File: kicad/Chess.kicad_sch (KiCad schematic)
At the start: 71 parts, among them J2 Conn_01x08_Pin, U1 CD74HC4067M, U12 A1302xUA, U13 A1302xUA, U14 A1302xUA, U15 A1302xUA, U16 A1302xUA, U17 A1302xUA, U18 A1302xUA, U19 A1302xUA, U2 ADS1015IDGS, U20 A1302xUA, U21 A1302xUA, U22 A1302xUA, U23 A1302xUA, U24 A1302xUA, U25 A1302xUA, U26 A1302xUA, U27 A1302xUA, U28 A1302xUA, U29 A1302xUA, U3 MP1584EN, U30 A1302xUA, U31 A1302xUA, U32 A1302xUA, U33 A1302xUA, U34 A1302xUA, U35 A1302xUA, U36 A1302xUA, U37 A1302xUA, U38 A1302xUA, U39 A1302xUA, U4 CD74HC4067M, U40 A1302xUA, U41 A1302xUA, U42 A1302xUA, U43 A1302xUA, U44 A1302xUA, U45 A1302xUA, U46 A1302xUA, U47 A1302xUA, U48 A1302xUA, U49 A1302xUA, U5 CD74HC4067M, U50 A1302xUA, U51 A1302xUA, U52 A1302xUA, U53 A1302xUA, U54 A1302xUA, U55 A1302xUA, U56 A1302xUA, U57 A1302xUA, U58 A1302xUA, U59 A1302xUA, U6 CD74HC4067M, U60 A1302xUA, U61 A1302xUA, U62 A1302xUA, U63 A1302xUA, U64 A1302xUA, U65 A1302xUA, U66 A1302xUA, U67 A1302xUA, U68 A1302xUA, U69 A1302xUA, U70 A1302xUA, U71 A1302xUA, U72 A1302xUA, U73 A1302xUA, U74 A1302xUA, U75 A1302xUA

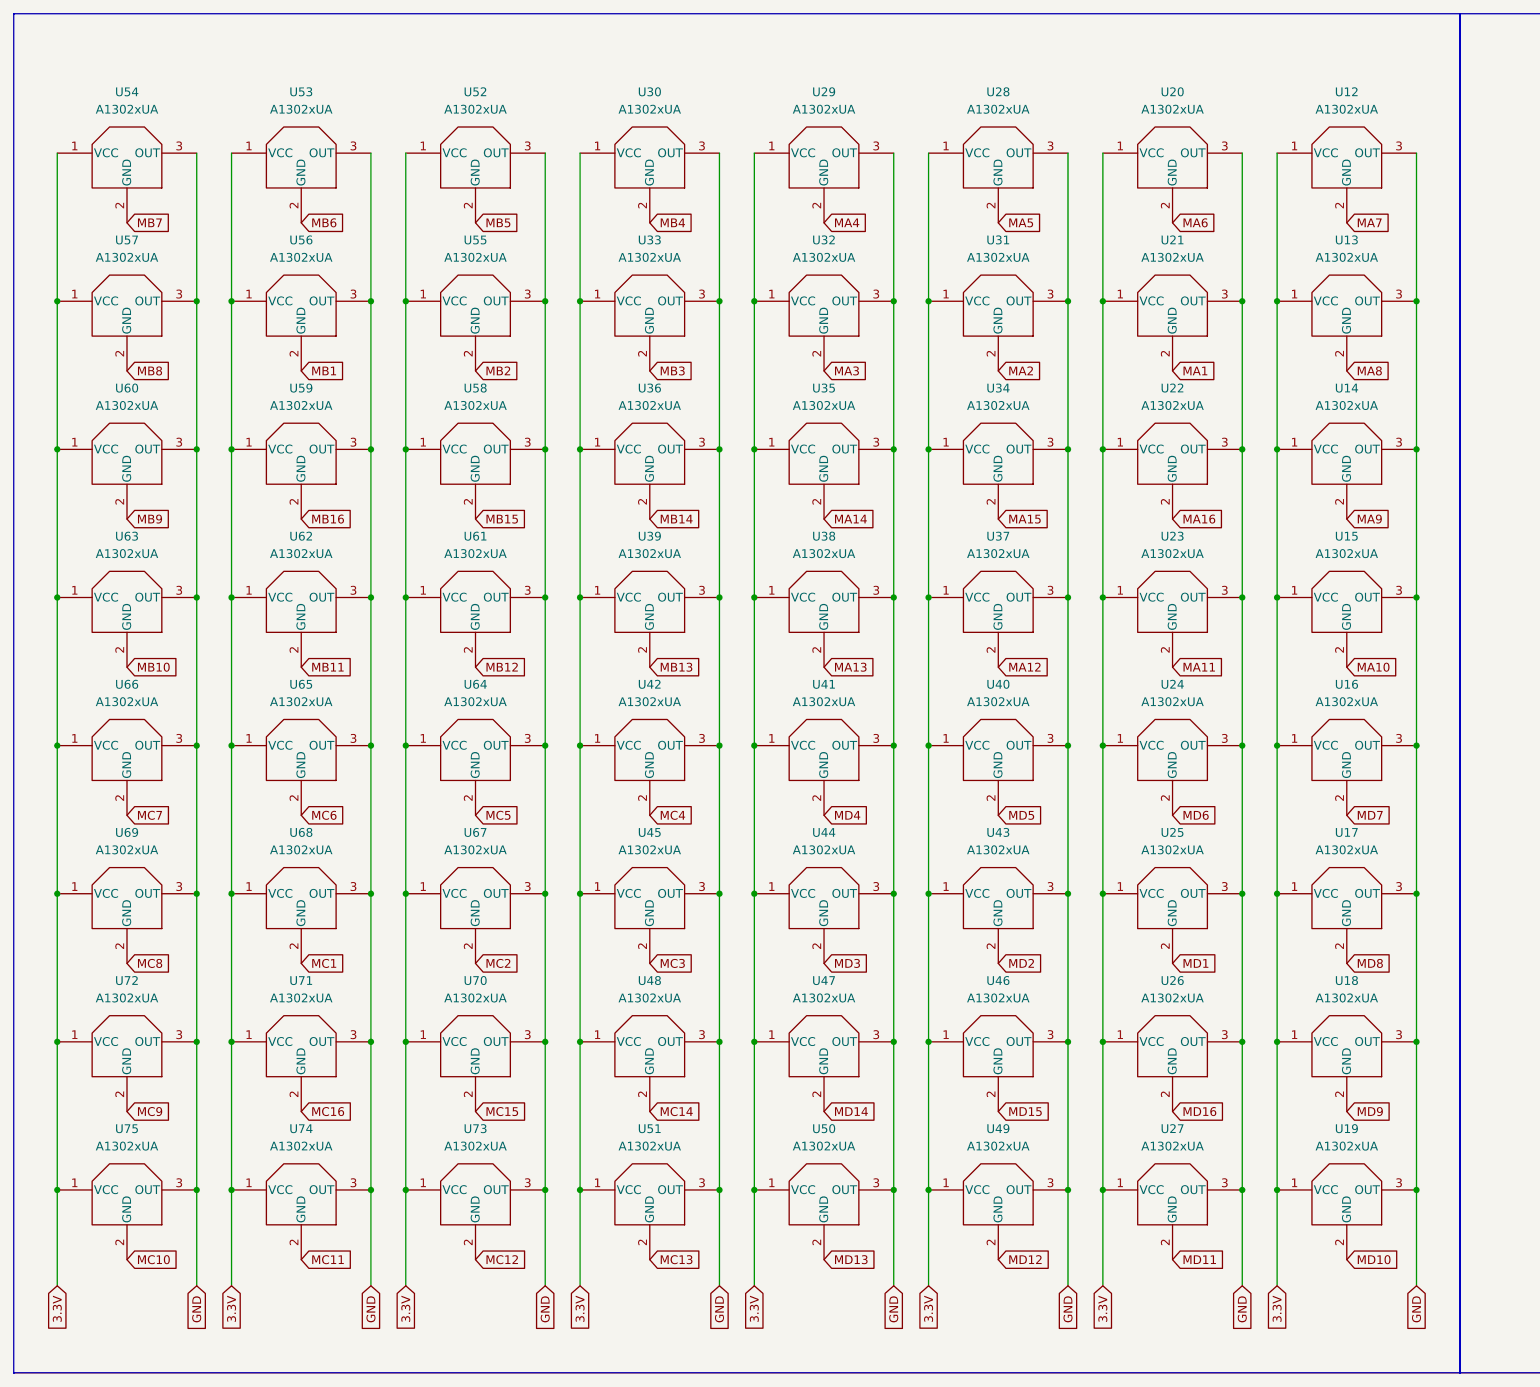
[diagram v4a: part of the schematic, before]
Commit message: fixes
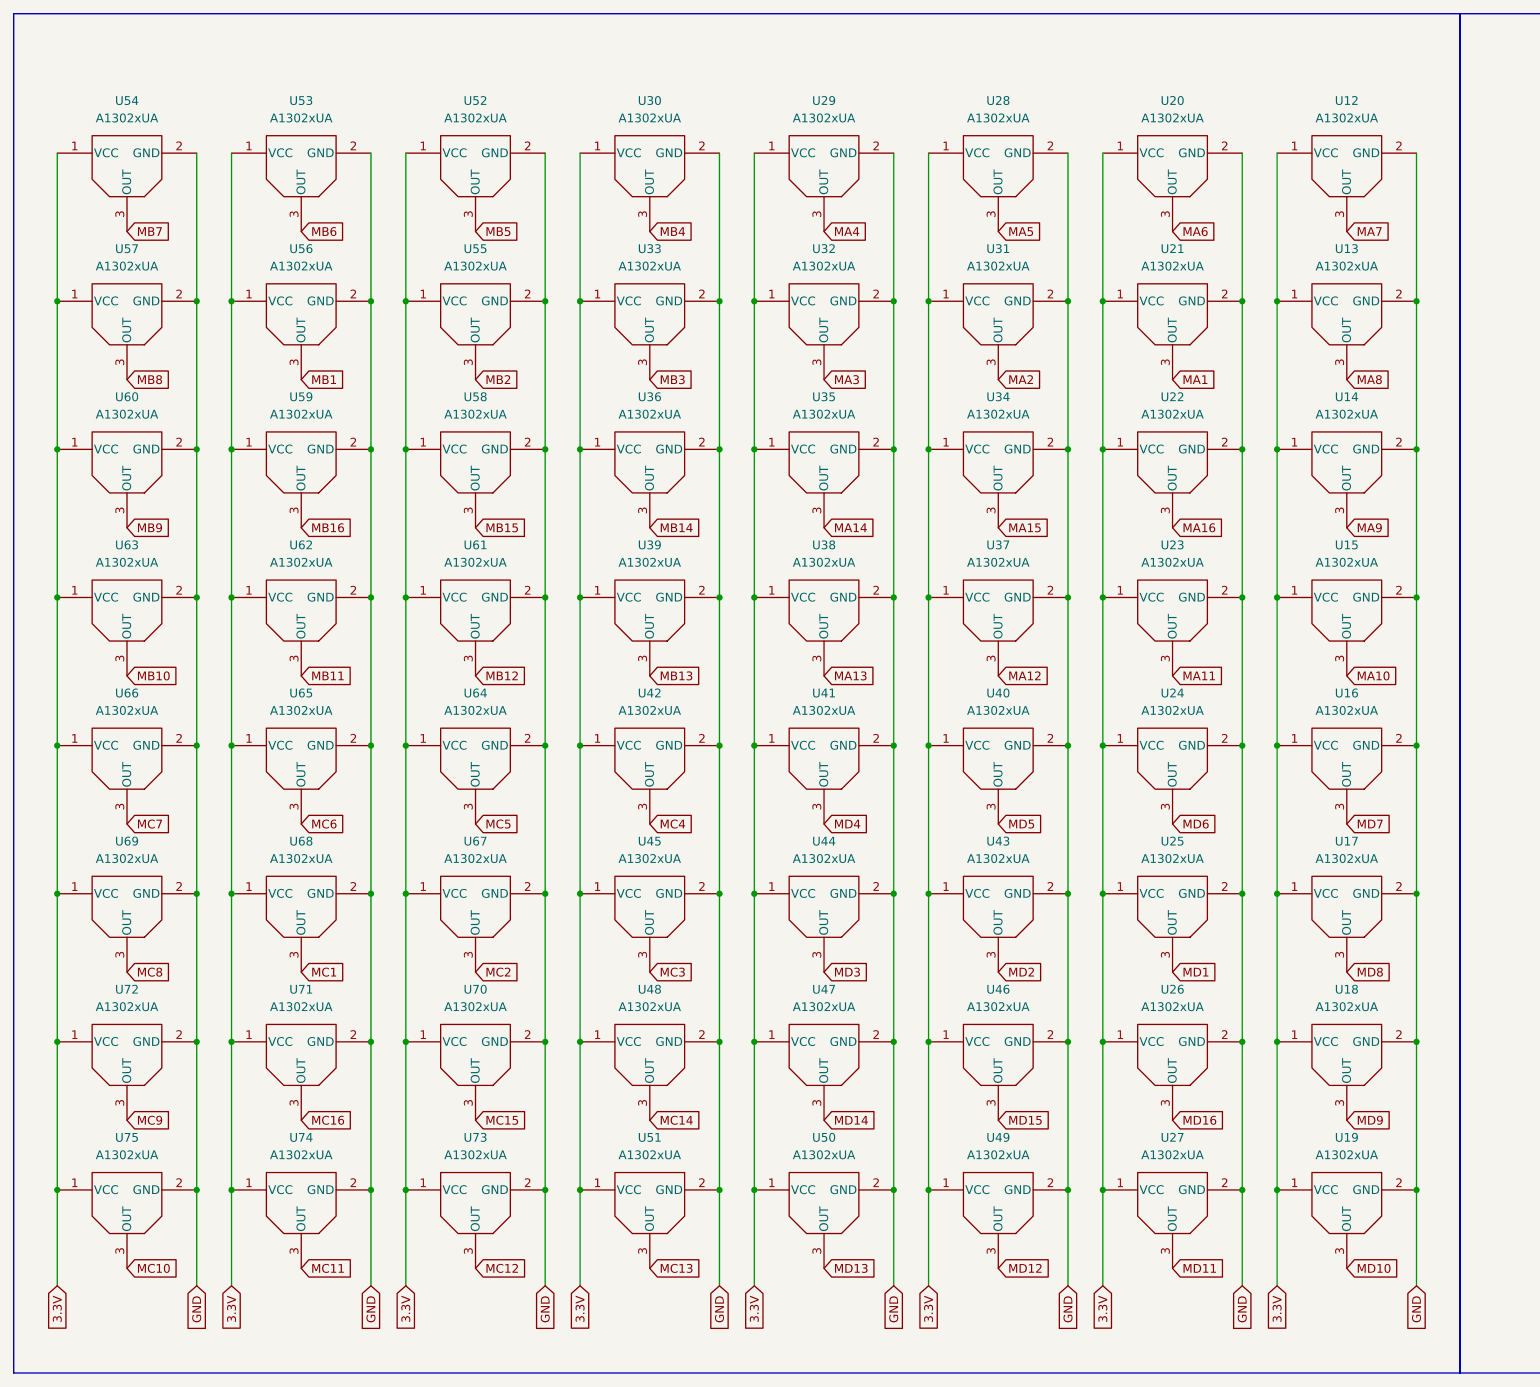
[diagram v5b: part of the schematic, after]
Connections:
- net GND: now also U12.2 (GND), U13.2 (GND), U14.2 (GND), U15.2 (GND), U16.2 (GND), U17.2 (GND), U18.2 (GND), U19.2 (GND), U20.2 (GND), U21.2 (GND), U22.2 (GND), U23.2 (GND), U24.2 (GND), U25.2 (GND), U26.2 (GND), U27.2 (GND), U28.2 (GND), U29.2 (GND), U30.2 (GND), U31.2 (GND), U32.2 (GND), U33.2 (GND), U34.2 (GND), U35.2 (GND), U36.2 (GND), U37.2 (GND), U38.2 (GND), U39.2 (GND), U40.2 (GND), U41.2 (GND), U42.2 (GND), U43.2 (GND), U44.2 (GND), U45.2 (GND), U46.2 (GND), U47.2 (GND), U48.2 (GND), U49.2 (GND), U50.2 (GND), U51.2 (GND), U52.2 (GND), U53.2 (GND), U54.2 (GND), U55.2 (GND), U56.2 (GND), U57.2 (GND), U58.2 (GND), U59.2 (GND), U60.2 (GND), U61.2 (GND), U62.2 (GND), U63.2 (GND), U64.2 (GND), U65.2 (GND), U66.2 (GND), U67.2 (GND), U68.2 (GND), U69.2 (GND), U70.2 (GND), U71.2 (GND), U72.2 (GND), U73.2 (GND), U74.2 (GND), U75.2 (GND); no longer U12.3 (OUT), U13.3 (OUT), U14.3 (OUT), U15.3 (OUT), U16.3 (OUT), U17.3 (OUT), U18.3 (OUT), U19.3 (OUT), U20.3 (OUT), U21.3 (OUT), U22.3 (OUT), U23.3 (OUT), U24.3 (OUT), U25.3 (OUT), U26.3 (OUT), U27.3 (OUT), U28.3 (OUT), U29.3 (OUT), U30.3 (OUT), U31.3 (OUT), U32.3 (OUT), U33.3 (OUT), U34.3 (OUT), U35.3 (OUT), U36.3 (OUT), U37.3 (OUT), U38.3 (OUT), U39.3 (OUT), U40.3 (OUT), U41.3 (OUT), U42.3 (OUT), U43.3 (OUT), U44.3 (OUT), U45.3 (OUT), U46.3 (OUT), U47.3 (OUT), U48.3 (OUT), U49.3 (OUT), U50.3 (OUT), U51.3 (OUT), U52.3 (OUT), U53.3 (OUT), U54.3 (OUT), U55.3 (OUT), U56.3 (OUT), U57.3 (OUT), U58.3 (OUT), U59.3 (OUT), U60.3 (OUT), U61.3 (OUT), U62.3 (OUT), U63.3 (OUT), U64.3 (OUT), U65.3 (OUT), U66.3 (OUT), U67.3 (OUT), U68.3 (OUT), U69.3 (OUT), U70.3 (OUT), U71.3 (OUT), U72.3 (OUT), U73.3 (OUT), U74.3 (OUT), U75.3 (OUT)
- net MA1: now also U21.3 (OUT); no longer U21.2 (GND)
- net MA10: now also U15.3 (OUT); no longer U15.2 (GND)
- net MA11: now also U23.3 (OUT); no longer U23.2 (GND)
- net MA12: now also U37.3 (OUT); no longer U37.2 (GND)
- net MA13: now also U38.3 (OUT); no longer U38.2 (GND)
- net MA14: now also U35.3 (OUT); no longer U35.2 (GND)
- net MA15: now also U34.3 (OUT); no longer U34.2 (GND)
- net MA16: now also U22.3 (OUT); no longer U22.2 (GND)
- net MA2: now also U31.3 (OUT); no longer U31.2 (GND)
- net MA3: now also U32.3 (OUT); no longer U32.2 (GND)
- net MA4: now also U29.3 (OUT); no longer U29.2 (GND)
- net MA5: now also U28.3 (OUT); no longer U28.2 (GND)
- net MA6: now also U20.3 (OUT); no longer U20.2 (GND)
- net MA7: now also U12.3 (OUT); no longer U12.2 (GND)
- net MA8: now also U13.3 (OUT); no longer U13.2 (GND)
- net MA9: now also U14.3 (OUT); no longer U14.2 (GND)
- net MB1: now also U56.3 (OUT); no longer U56.2 (GND)
- net MB10: now also U63.3 (OUT); no longer U63.2 (GND)
- net MB11: now also U62.3 (OUT); no longer U62.2 (GND)
- net MB12: now also U61.3 (OUT); no longer U61.2 (GND)
- net MB13: now also U39.3 (OUT); no longer U39.2 (GND)
- net MB14: now also U36.3 (OUT); no longer U36.2 (GND)
- net MB15: now also U58.3 (OUT); no longer U58.2 (GND)
- net MB16: now also U59.3 (OUT); no longer U59.2 (GND)
- net MB2: now also U55.3 (OUT); no longer U55.2 (GND)
- net MB3: now also U33.3 (OUT); no longer U33.2 (GND)
- net MB4: now also U30.3 (OUT); no longer U30.2 (GND)
- net MB5: now also U52.3 (OUT); no longer U52.2 (GND)
- net MB6: now also U53.3 (OUT); no longer U53.2 (GND)
- net MB7: now also U54.3 (OUT); no longer U54.2 (GND)
- net MB8: now also U57.3 (OUT); no longer U57.2 (GND)
- net MB9: now also U60.3 (OUT); no longer U60.2 (GND)
- net MC1: now also U68.3 (OUT); no longer U68.2 (GND)
- net MC10: now also U75.3 (OUT); no longer U75.2 (GND)
- net MC11: now also U74.3 (OUT); no longer U74.2 (GND)
- net MC12: now also U73.3 (OUT); no longer U73.2 (GND)
- net MC13: now also U51.3 (OUT); no longer U51.2 (GND)
- net MC14: now also U48.3 (OUT); no longer U48.2 (GND)
- net MC15: now also U70.3 (OUT); no longer U70.2 (GND)
- net MC16: now also U71.3 (OUT); no longer U71.2 (GND)
- net MC2: now also U67.3 (OUT); no longer U67.2 (GND)
- net MC3: now also U45.3 (OUT); no longer U45.2 (GND)
- net MC4: now also U42.3 (OUT); no longer U42.2 (GND)
- net MC5: now also U64.3 (OUT); no longer U64.2 (GND)
- net MC6: now also U65.3 (OUT); no longer U65.2 (GND)
- net MC7: now also U66.3 (OUT); no longer U66.2 (GND)
- net MC8: now also U69.3 (OUT); no longer U69.2 (GND)
- net MC9: now also U72.3 (OUT); no longer U72.2 (GND)
- net MD1: now also U25.3 (OUT); no longer U25.2 (GND)
- net MD10: now also U19.3 (OUT); no longer U19.2 (GND)
- net MD11: now also U27.3 (OUT); no longer U27.2 (GND)
- net MD12: now also U49.3 (OUT); no longer U49.2 (GND)
- net MD13: now also U50.3 (OUT); no longer U50.2 (GND)
- net MD14: now also U47.3 (OUT); no longer U47.2 (GND)
- net MD15: now also U46.3 (OUT); no longer U46.2 (GND)
- net MD16: now also U26.3 (OUT); no longer U26.2 (GND)
- net MD2: now also U43.3 (OUT); no longer U43.2 (GND)
- net MD3: now also U44.3 (OUT); no longer U44.2 (GND)
- net MD4: now also U41.3 (OUT); no longer U41.2 (GND)
- net MD5: now also U40.3 (OUT); no longer U40.2 (GND)
- net MD6: now also U24.3 (OUT); no longer U24.2 (GND)
- net MD7: now also U16.3 (OUT); no longer U16.2 (GND)
- net MD8: now also U17.3 (OUT); no longer U17.2 (GND)
- net MD9: now also U18.3 (OUT); no longer U18.2 (GND)
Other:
- moved on the sheet: U12, U13, U14, U15, U16, U17, U18, U19, U20, U21, U22, U23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
